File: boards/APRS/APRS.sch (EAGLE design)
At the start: 15 parts

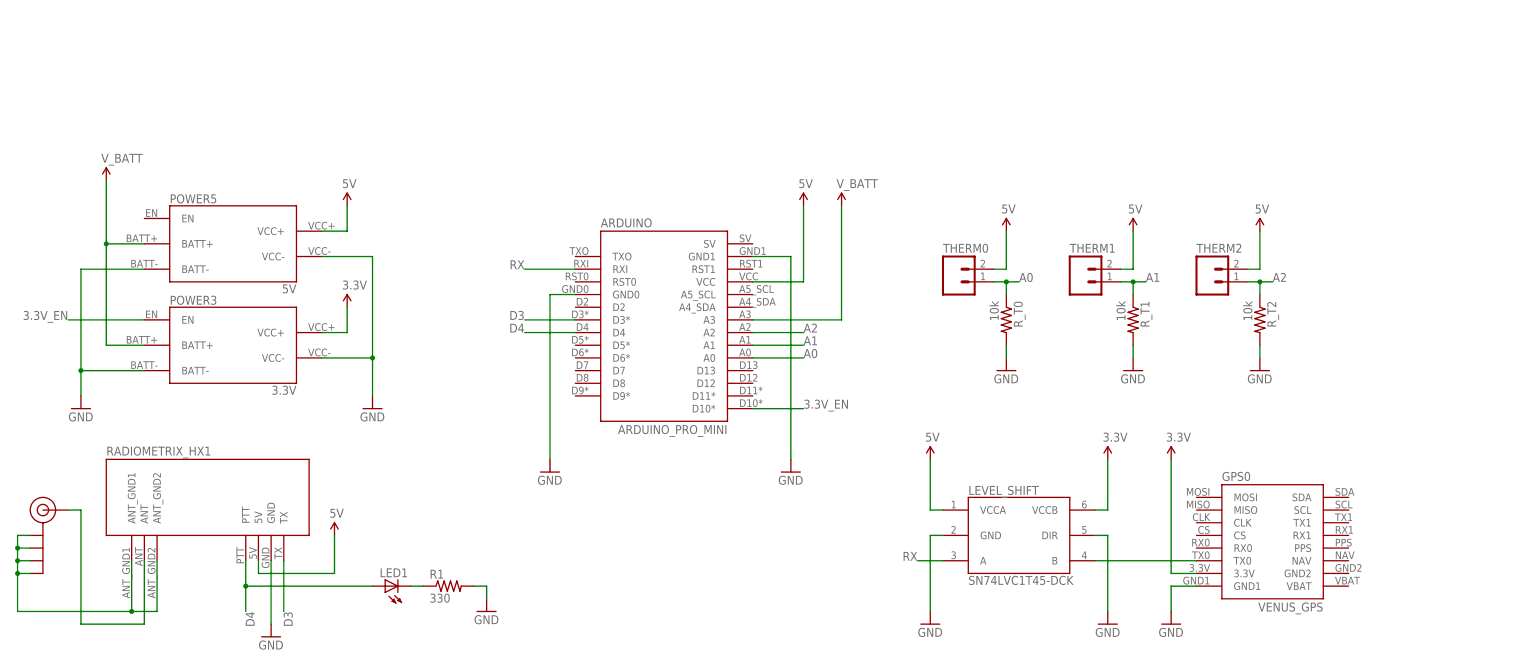
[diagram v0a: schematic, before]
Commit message: New APRS board, close to ready
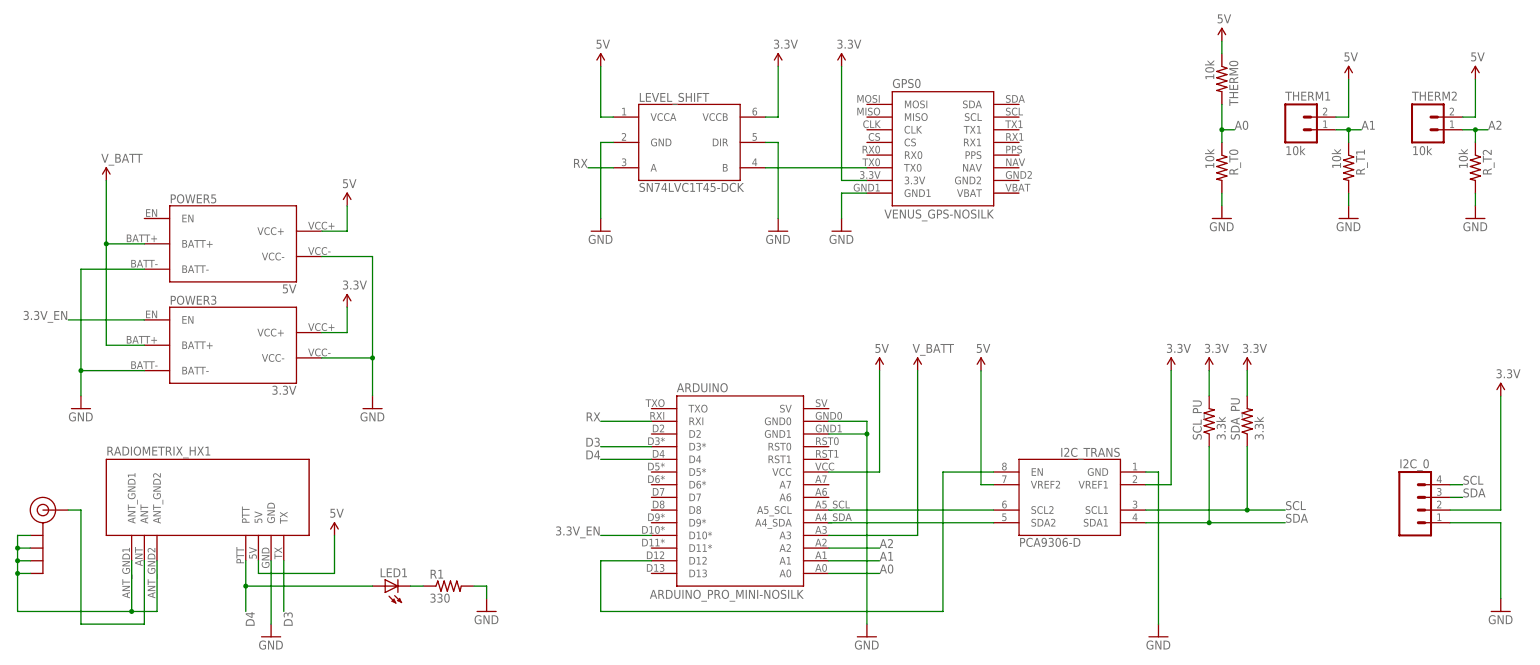
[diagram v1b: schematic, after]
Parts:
- added I2C_0: (no value), SparkFun-Connectors:M04PTH
- added I2C_TRANS: PCA9306-D, OpenSpace:PCA9306-D
- added SCL_PU, SDA_PU: 3.3k, SparkFun-Passives:RESISTOR0805-RES
- ARDUINO: value ARDUINO_PRO_MINI -> ARDUINO_PRO_MINI-NOSILK; device OpenSpace:ARDUINO_PRO_MINI -> OpenSpace:ARDUINO_PRO_MINI-NOSILK
- GPS0: value VENUS_GPS -> VENUS_GPS-NOSILK; device OpenSpace:VENUS_GPS -> OpenSpace:VENUS_GPS-NOSILK
- POWER3, POWER5: device OpenSpace:POWER-TPS6300X -> OpenSpace:POWER-TPS6300X-NOSILK
- THERM0: value (none) -> 10k; device SparkFun:M02PTH -> SparkFun-Passives:RESISTOR0805-RES
- THERM1, THERM2: value (none) -> 10k
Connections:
- new net N$4: ARDUINO.A4_SDA, I2C_TRANS.SDA2
- new net N$5: ARDUINO.A5_SCL, I2C_TRANS.SCL2
- new net N$6: ARDUINO.D12, I2C_TRANS.EN
- new net SCL: I2C_0.4, I2C_TRANS.SCL1, SDA_PU.1
- new net SDA: I2C_0.3, I2C_TRANS.SDA1, SCL_PU.1
- net 3.3V: now also I2C_0.2, I2C_TRANS.VREF1, SCL_PU.2, SDA_PU.2
- net 5V: now also I2C_TRANS.VREF2, THERM0.1; no longer THERM0.2
- net A0: now also THERM0.2; no longer THERM0.1
- net GND: now also I2C_0.1, I2C_TRANS.GND
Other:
- moved on the sheet: GPS0, LEVEL_SHIFT, R_T0, R_T1, R_T2, THERM1, THERM2
